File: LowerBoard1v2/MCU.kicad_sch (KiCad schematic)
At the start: 109 parts, among them J401 PWR, J402 DATA, J403 SWD Header, J404 MIDI_In, J405 Micro_SD_Card_Det2, J406 MIDI_Out, J407 MIDI_Thru, J408 POWER, Q401 2N7002H, Q402 2N7002H, SW401 RST, SW402 BOOT, U401 STM32F411RET6, U402 TPS56528DDA, U403 AMS1117, U404 74HC04, U405 6N138, Y401 16MHz, Y402 32.768kHZ

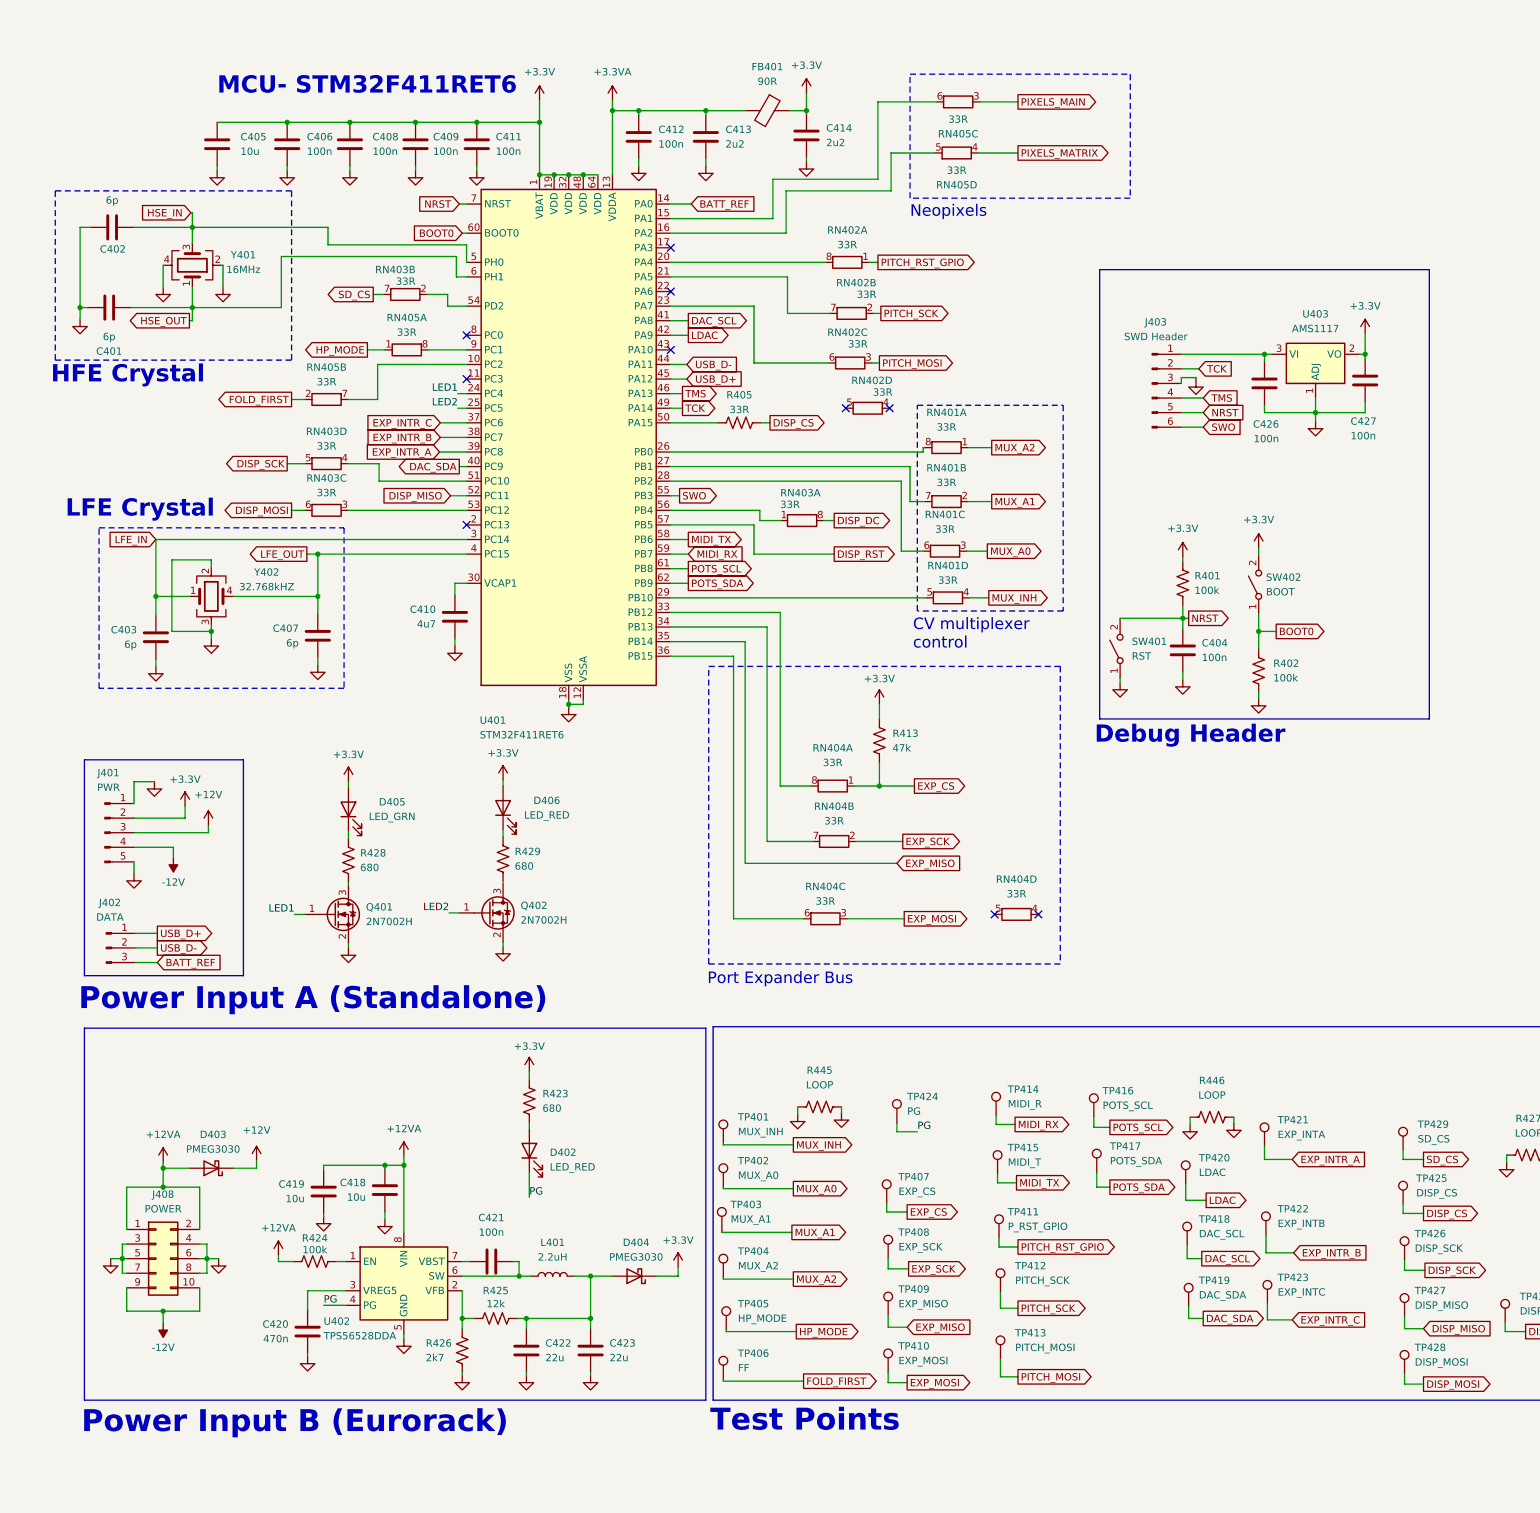
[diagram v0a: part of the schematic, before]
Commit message: power supply and load switch stuff
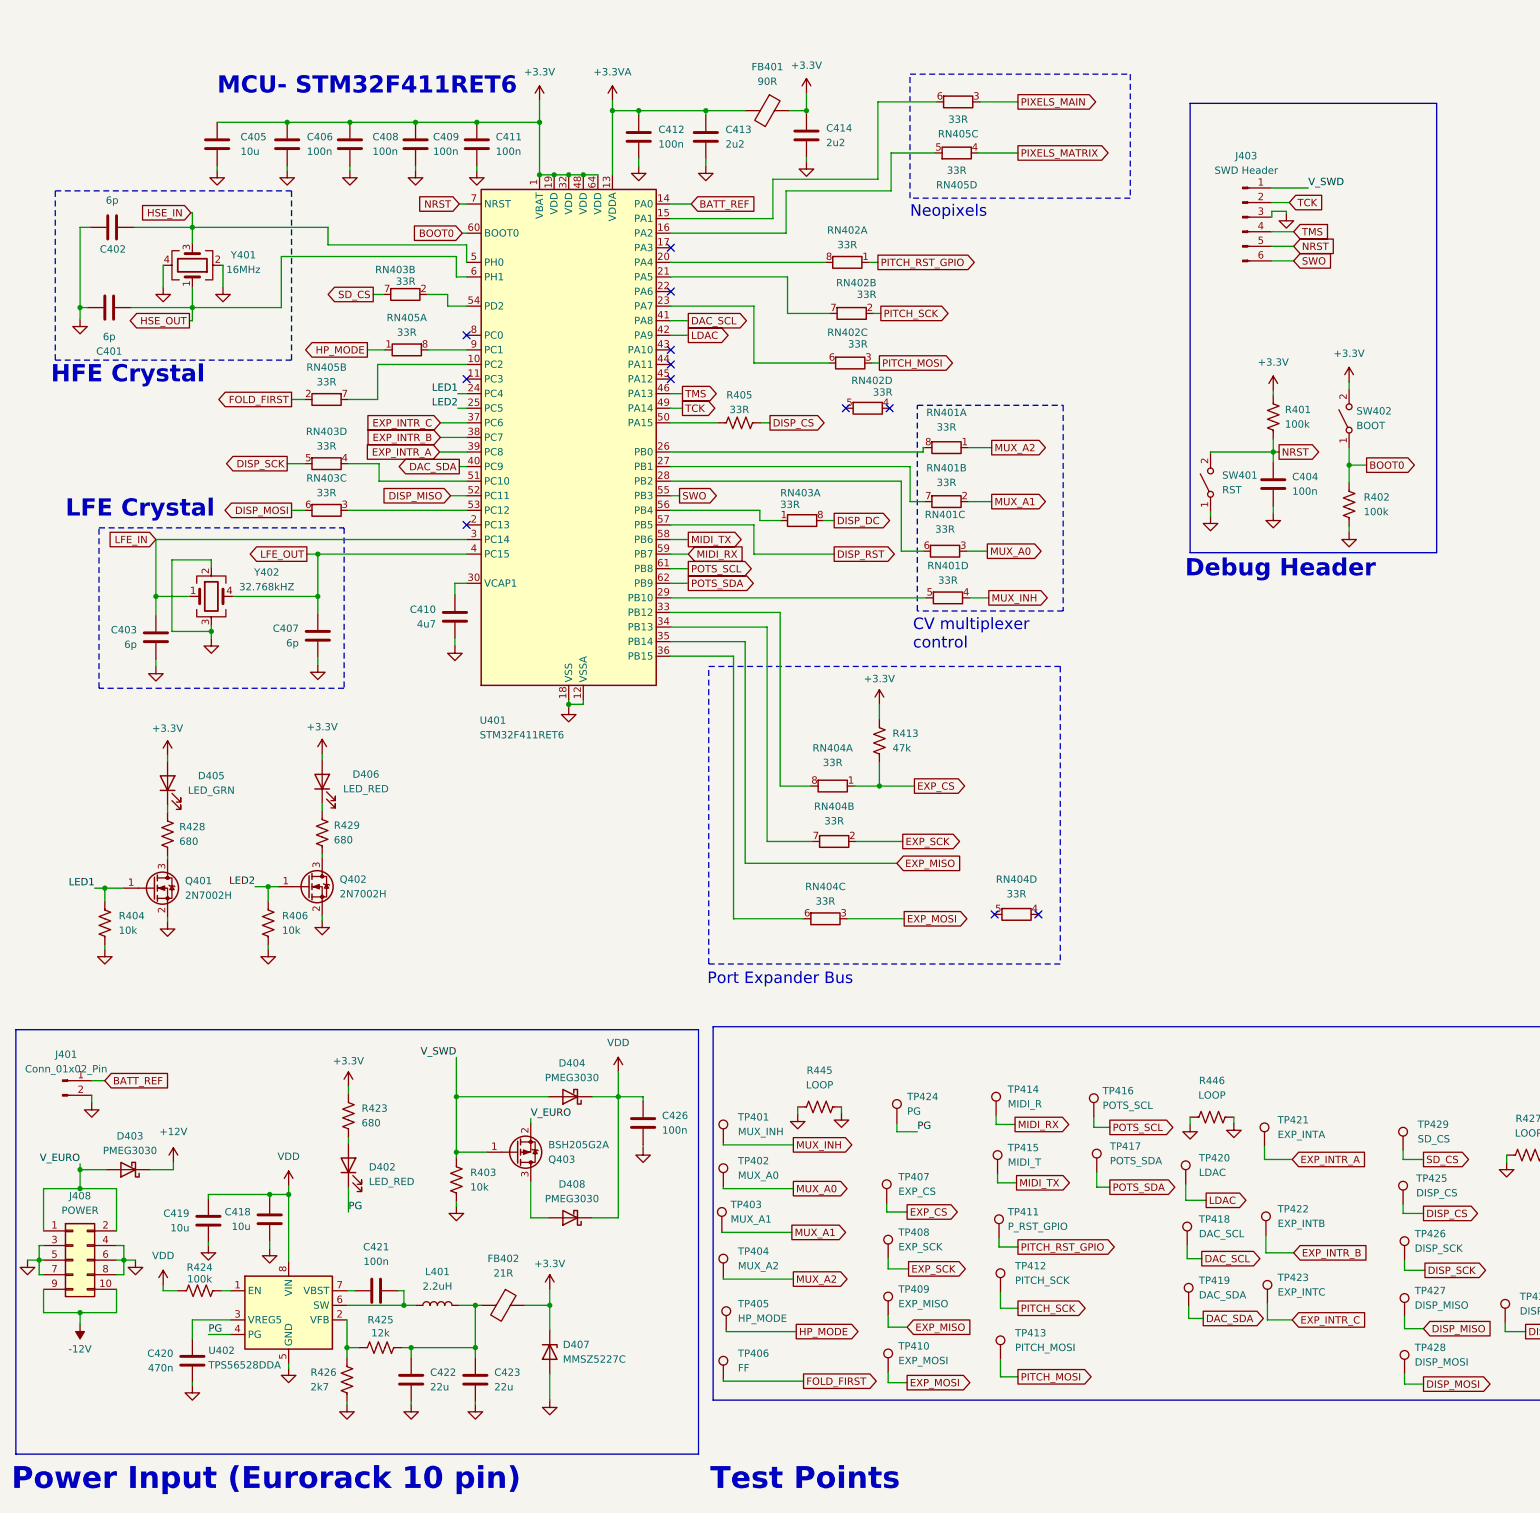
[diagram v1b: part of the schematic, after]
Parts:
- removed C427: 100n, Capacitor_SMD:C_0805_2012Metric, symbol Device:C
- removed J401: PWR, Connector_PinHeader_2.54mm:PinHeader_1x05_P2.54mm_Vertical, symbol Connector:Conn_01x05_Pin
- removed J402: DATA, Connector_PinHeader_2.54mm:PinHeader_1x03_P2.54mm_Vertical, symbol Connector:Conn_01x03_Pin
- removed U403: AMS1117, Package_TO_SOT_SMD:SOT-223-3_TabPin2, symbol Regulator_Linear:AMS1117
- added D407: MMSZ5227C, Diode_SMD:D_SOD-123, symbol Device:D_Zener
- added D408: PMEG3030, Diode_SMD:D_SOD-123, symbol Device:D_Schottky
- added FB402: 21R, Inductor_SMD:L_0805_2012Metric, symbol Device:FerriteBead
- added J401: Conn_01x02_Pin, Connector_PinHeader_2.54mm:PinHeader_1x02_P2.54mm_Vertical, symbol Connector:Conn_01x02_Pin
- added Q403: BSH205G2A, PCM_4ms_Package_SOT:SOT-23, symbol Device:Q_PMOS_GSD
- added R403, R404, R406: 10k, Resistor_SMD:R_0805_2012Metric, symbol Device:R_US
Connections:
- net +3.3V: now also D407.1 (K), FB402.1; no longer D404.1 (K)
- net BATT_REF: now also J401.1 (Pin_1)
- net GND: now also C426.2, D407.2 (A), J401.2 (Pin_2), R403.2, R404.2, R406.2; no longer C426.1
- net LED1: now also R404.1
- net LED2: now also R406.1
- net at C422.1, C423.1, L401.2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: now also FB402.2; no longer D404.2 (A)
- net V_SWD: now reaches J403.1 (Pin_1)
- net V_SWD: now also D404.2 (A), Q403.1 (G), R403.1; no longer C426.2
- net +12VA renamed VDD
- net VDD: now also C426.1, D404.1 (K), D408.1 (K); no longer D403.2 (A), J408.1 (Pin_1), J408.2 (Pin_2)
- net USB_D+: no longer names the net of U401.45 (PA12)
- net USB_D-: no longer names the net of U401.44 (PA11)
- new net: D408.2 (A), Q403.3 (D)
- new net V_EURO: D403.2 (A), J408.1 (Pin_1), J408.2 (Pin_2), Q403.2 (S)
- no-connect marks 18 -> 20
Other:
- note added: "Power Input (Eurorack 10 pin)"
- note removed: "Power Input A (Standalone)"
- note removed: "Power Input B (Eurorack)"
- moved on the sheet: C404, C418, C419, C420, C421, C422, C423, D402, D403, D405, D406, J403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
